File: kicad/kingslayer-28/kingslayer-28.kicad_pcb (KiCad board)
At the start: 2 copper layers, 133 x 95 mm, 119 parts, among them IC1 STM32F303CCT7, IC2 IS31FL3731-QFLS2-TR, IC3 LM3940IMP-3.3_NOPB, J1 Conn_01x04_Pin, K1 KEYSW, K10 KEYSW, K11 KEYSW, K12 KEYSW, K13 KEYSW, K14 KEYSW, K15 KEYSW, K16 KEYSW, K17 KEYSW, K18 KEYSW, K19 KEYSW, K2 KEYSW, K20 KEYSW, K21 KEYSW, K22 KEYSW, K24 KEYSW, K25 KEYSW, K26 KEYSW, K27 KEYSW, K28 KEYSW, K3 KEYSW, K4 KEYSW, K5 KEYSW, K6 KEYSW, K7 KEYSW, K8 KEYSW, K9 KEYSW, SW1 SS12D07, X1 IC21008.000M30.0EE1B

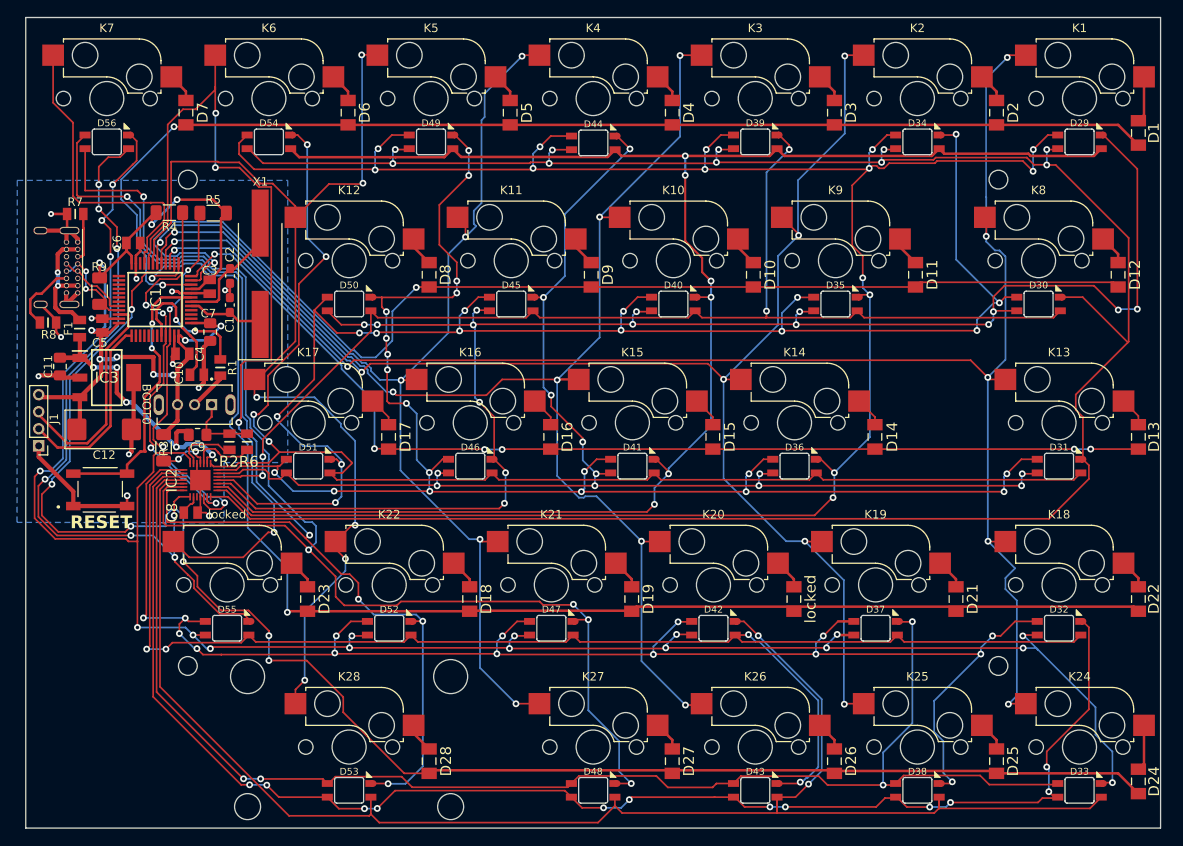
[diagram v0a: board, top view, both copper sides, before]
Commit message: fix RGB
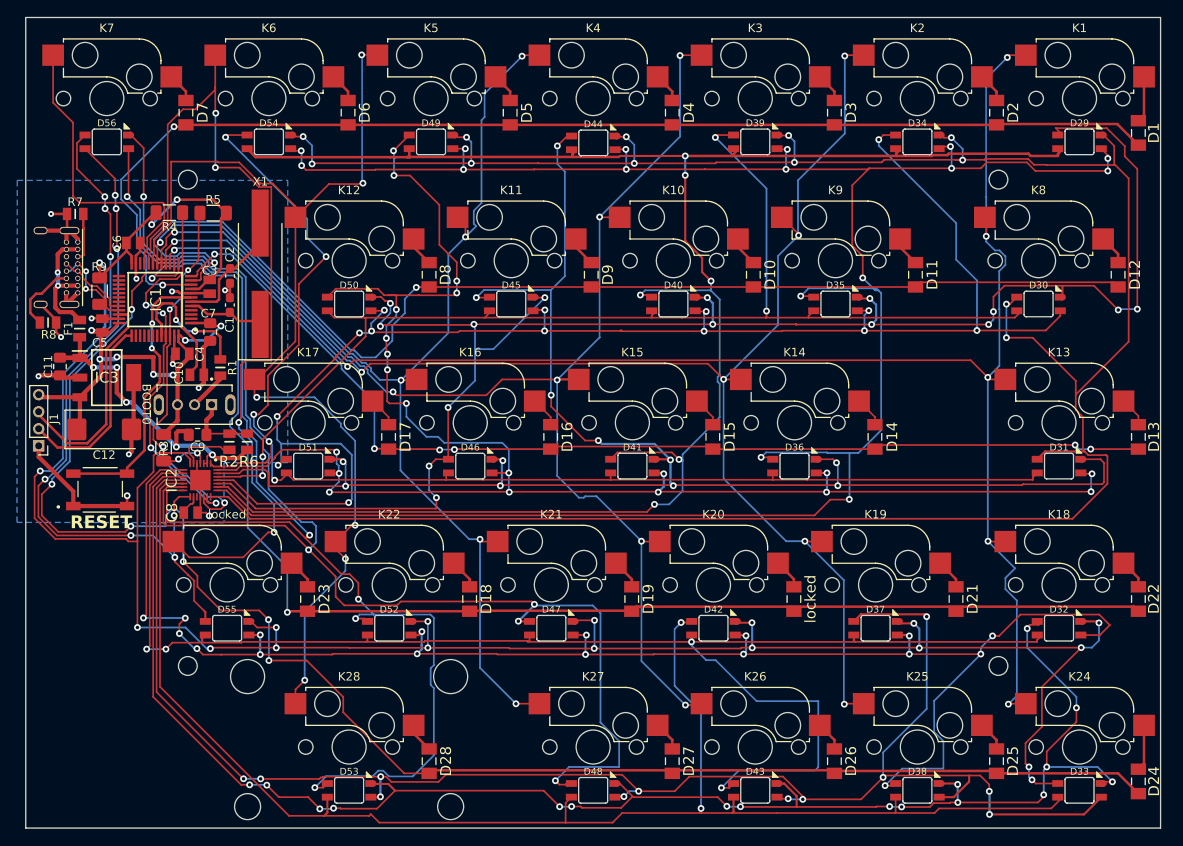
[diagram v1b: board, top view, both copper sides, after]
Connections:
- D29 pad 1: ca1 -> ca3
- D29 pad 2: ca2 -> ca4
- D29 pad 3: ca3 -> ca2
- D29 pad 4: ca4 -> ca1
- D30 pad 1: ca4 -> ca6
- D30 pad 2: ca5 -> ca1
- D30 pad 3: ca6 -> ca5
- D30 pad 4: ca1 -> ca4
- D31 pad 1: ca7 -> ca9
- D31 pad 2: ca8 -> ca1
- D31 pad 3: ca9 -> ca8
- D31 pad 4: ca1 -> ca7
- D32 pad 1: cb1 -> cb3
- D32 pad 2: cb2 -> cb4
- D32 pad 3: cb3 -> cb2
- D32 pad 4: cb4 -> cb1
- D33 pad 1: cb4 -> cb6
- D33 pad 2: cb5 -> cb1
- D33 pad 3: cb6 -> cb5
- D33 pad 4: cb1 -> cb4
- D34 pad 1: ca1 -> ca3
- D34 pad 2: ca2 -> ca5
- D34 pad 3: ca3 -> ca2
- D34 pad 4: ca5 -> ca1
- D35 pad 1: ca4 -> ca6
- D35 pad 2: ca5 -> ca2
- D35 pad 3: ca6 -> ca5
- D35 pad 4: ca2 -> ca4
- D36 pad 1: ca7 -> ca9
- D36 pad 2: ca8 -> ca2
- D36 pad 3: ca9 -> ca8
- D36 pad 4: ca2 -> ca7
- D37 pad 1: cb1 -> cb3
- D37 pad 2: cb2 -> cb5
- D37 pad 3: cb3 -> cb2
- D37 pad 4: cb5 -> cb1
- D38 pad 1: cb4 -> cb6
- D38 pad 2: cb5 -> cb2
- D38 pad 3: cb6 -> cb5
- D38 pad 4: cb2 -> cb4
- D39 pad 1: ca1 -> ca3
- D39 pad 2: ca2 -> ca6
- D39 pad 3: ca3 -> ca2
- D39 pad 4: ca6 -> ca1
- D40 pad 1: ca4 -> ca6
- D40 pad 2: ca5 -> ca3
- D40 pad 3: ca6 -> ca5
- D40 pad 4: ca3 -> ca4
- D41 pad 1: ca7 -> ca9
- D41 pad 2: ca8 -> ca3
- D41 pad 3: ca9 -> ca8
- D41 pad 4: ca3 -> ca7
- D42 pad 1: cb1 -> cb3
- D42 pad 2: cb2 -> cb6
- D42 pad 3: cb3 -> cb2
- D42 pad 4: cb6 -> cb1
- D43 pad 1: cb4 -> cb6
- D43 pad 2: cb5 -> cb3
- D43 pad 3: cb6 -> cb5
- D43 pad 4: cb3 -> cb4
- D44 pad 1: ca1 -> ca3
- D44 pad 2: ca2 -> ca7
- D44 pad 3: ca3 -> ca2
- D44 pad 4: ca7 -> ca1
- D45 pad 1: ca4 -> ca6
- D45 pad 2: ca5 -> ca7
- D45 pad 3: ca6 -> ca5
- D45 pad 4: ca7 -> ca4
- D46 pad 1: ca7 -> ca9
- D46 pad 2: ca8 -> ca4
- D46 pad 3: ca9 -> ca8
- D46 pad 4: ca4 -> ca7
- D47 pad 1: cb1 -> cb3
- D47 pad 2: cb2 -> cb7
- D47 pad 3: cb3 -> cb2
- D47 pad 4: cb7 -> cb1
- D48 pad 1: cb4 -> cb6
- D48 pad 2: cb5 -> cb7
- D48 pad 3: cb6 -> cb5
- D48 pad 4: cb7 -> cb4
- D49 pad 1: ca1 -> ca3
- D49 pad 2: ca2 -> ca8
- D49 pad 3: ca3 -> ca2
- D49 pad 4: ca8 -> ca1
- D50 pad 1: ca4 -> ca6
- D50 pad 2: ca5 -> ca8
- D50 pad 3: ca6 -> ca5
- D50 pad 4: ca8 -> ca4
- D51 pad 1: ca7 -> ca9
- D51 pad 2: ca8 -> ca5
- D51 pad 3: ca9 -> ca8
- D51 pad 4: ca5 -> ca7
- D52 pad 1: cb1 -> cb3
- D52 pad 2: cb2 -> cb8
- D52 pad 3: cb3 -> cb2
- D52 pad 4: cb8 -> cb1
- D53 pad 1: cb4 -> cb6
- D53 pad 2: cb5 -> cb8
- D53 pad 3: cb6 -> cb5
- D53 pad 4: cb8 -> cb4
- D54 pad 1: ca1 -> ca3
- D54 pad 2: ca2 -> ca9
- D54 pad 3: ca3 -> ca2
- D54 pad 4: ca9 -> ca1
- D55 pad 1: cb1 -> cb3
- D55 pad 2: cb2 -> cb9
- D55 pad 3: cb3 -> cb2
- D55 pad 4: cb9 -> cb1
- D56 pad 1: cb7 -> cb9
- D56 pad 2: cb8 -> cb1
- D56 pad 3: cb9 -> cb8
- D56 pad 4: cb1 -> cb7
- IC2 pad 3: sdb -> +5V
- R6 pad 1: sdb -> +5V
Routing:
- net ca7: track 156.4 -> 190.8 mm
- net cb5: track 164.0 -> 196.5 mm, vias 4 -> 12
- net ca1: track 272.6 -> 297.4 mm, vias 10 -> 12
- net ca8: track 175.1 -> 199.0 mm, vias 19 -> 20
- net cb4: track 168.0 -> 190.7 mm, vias 12 -> 17
- net ca3: track 200.2 -> 219.0 mm
- net cb1: track 238.7 -> 256.6 mm, vias 18 -> 20
- net cb3: track 163.6 -> 174.4 mm
- net ca4: track 193.1 -> 203.1 mm
- net ca2: track 250.2 -> 259.6 mm, vias 14 -> 16
- net cb6: track 183.1 -> 173.8 mm
- net cb2: track 179.8 -> 188.9 mm, vias 15 -> 17
- net sdb: track 7.35 -> 0.00 mm
- net cb8: track 134.1 -> 140.7 mm
- net cb7: track 155.3 -> 160.8 mm
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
